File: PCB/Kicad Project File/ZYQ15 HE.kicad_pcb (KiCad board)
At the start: 2 copper layers, 154.3 x 110.2 mm, 130 parts, among them J1 I2C OLED, U16 ESP32-S3-DevKitC

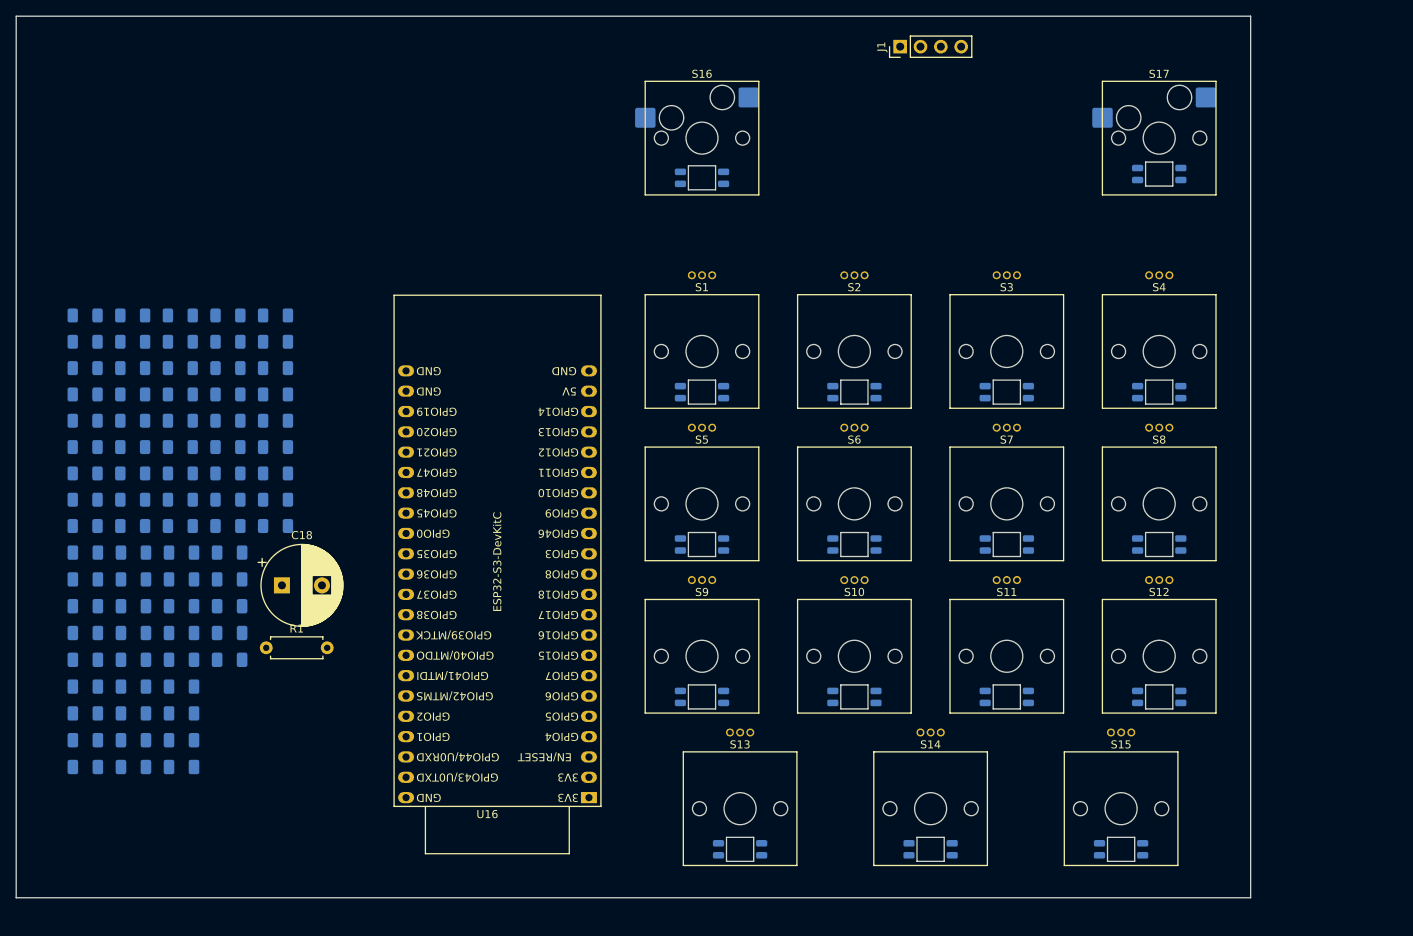
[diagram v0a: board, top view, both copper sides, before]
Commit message: Updated PCB Design files
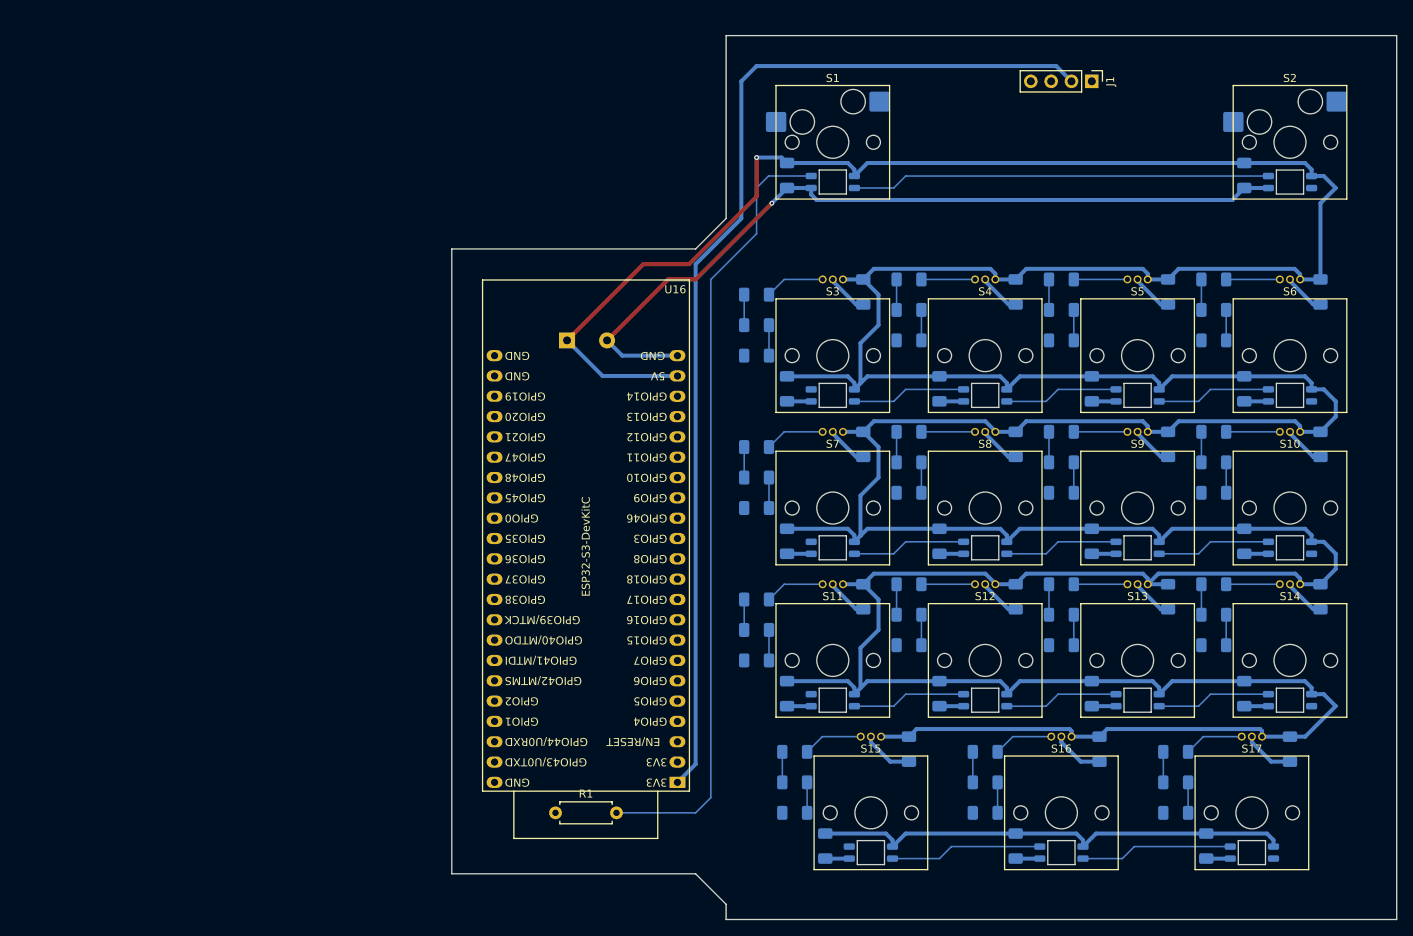
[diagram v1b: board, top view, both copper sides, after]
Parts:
- S1, S2: value HE Switch -> Keyswitch; footprint ScottoKeebs_MX:MX_HE_PCB_1.00u -> ScottoKeebs_Hotswap:Hotswap_MX_1.00u
- S13, S14: footprint ScottoKeebs_MX:MX_HE_PCB_1.25u -> ScottoKeebs_MX:MX_HE_PCB_1.00u
- S16, S17: value Keyswitch -> HE Switch; footprint ScottoKeebs_Hotswap:Hotswap_MX_1.00u -> ScottoKeebs_MX:MX_HE_PCB_1.25u
- moved C2 153.4 mm to (232.4, 44.2), turned to -90 degrees
- moved C6 149.6 mm to (232.4, 70.8), turned to -90 degrees
- moved C22 147.7 mm to (241.9, 58.7), turned to -90 degrees
- moved C26 146.3 mm to (241.9, 77.8), turned to -90 degrees
- moved C14 138.9 mm to (232.4, 108.9), turned to -90 degrees
- moved C10 138.9 mm to (232.4, 89.9), turned to -90 degrees
- moved C30 136.4 mm to (241.9, 96.8), turned to -90 degrees
- moved R11 135.2 mm to (228.6, 57.1)
- moved R12 135.2 mm to (228.6, 61.0)
- moved R13 135.2 mm to (228.6, 64.8)
- moved C17 134.8 mm to (227.7, 128.0), turned to -90 degrees
- moved C33 133.0 mm to (238.1, 115.9), turned to -90 degrees
- moved C5 130.3 mm to (213.4, 70.8), turned to -90 degrees
- moved R25 129.3 mm to (228.6, 83.8)
- moved R24 129.3 mm to (228.6, 80.0)
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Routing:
- net 5V: track 0.00 -> 737.0 mm, vias 0 -> 1
- net GND: track 0.00 -> 229.3 mm, vias 0 -> 1
- net 3.3V: track 0.00 -> 133.8 mm
- net Net-(D1-DIN): track 0.00 -> 98.6 mm
- net Net-(D1-DOUT): track 0.00 -> 52.4 mm
- net Net-(D16-DOUT): track 0.00 -> 19.0 mm
- net Net-(D15-DOUT): track 0.00 -> 19.0 mm
- net Net-(D8-DOUT): track 0.00 -> 14.3 mm
- net Net-(D5-DOUT): track 0.00 -> 14.3 mm
- net Net-(D4-DOUT): track 0.00 -> 14.3 mm
- net Net-(D13-DOUT): track 0.00 -> 14.3 mm
- net Net-(D12-DOUT): track 0.00 -> 14.3 mm
- net Net-(D10-DIN): track 0.00 -> 14.3 mm
- net Net-(D7-DOUT): track 0.00 -> 14.3 mm
- net Net-(D3-DOUT): track 0.00 -> 14.3 mm
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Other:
- board size 154.3 x 110.2 mm -> 118.1 x 110.5 mm
